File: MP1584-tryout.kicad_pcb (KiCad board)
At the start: 2 copper layers, 15 parts, among them J1 Conn_01x03_Female, U1 MP1584

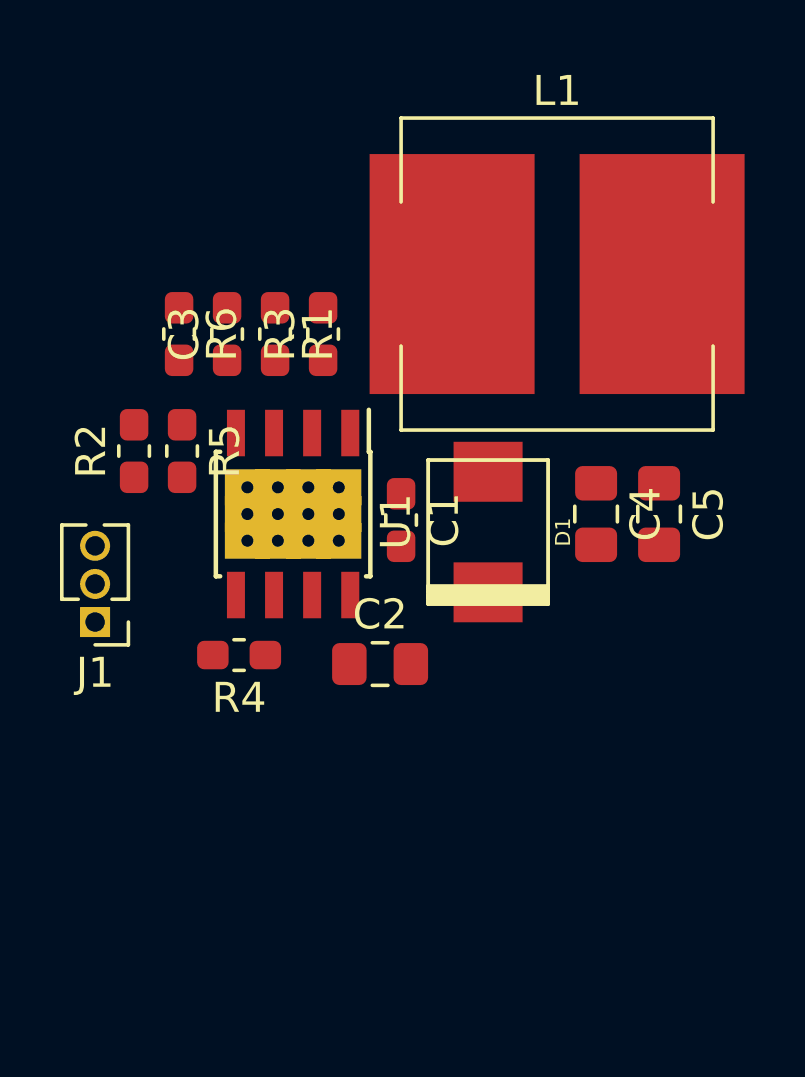
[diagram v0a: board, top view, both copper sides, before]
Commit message: final,
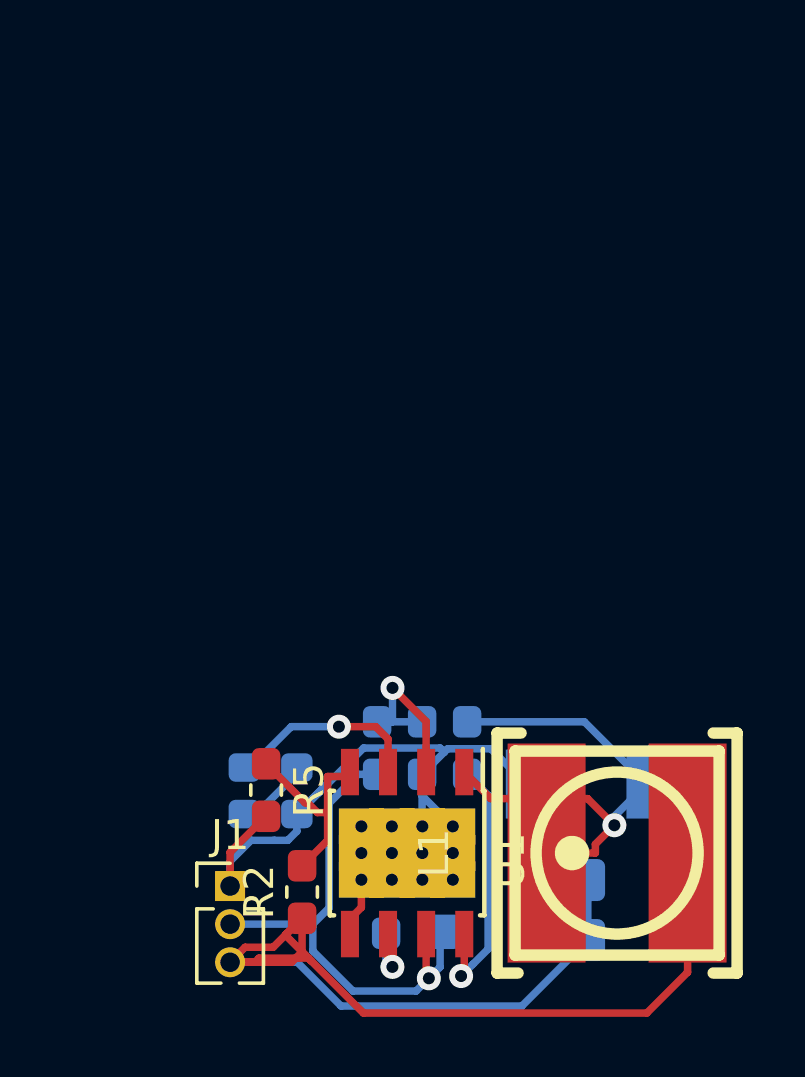
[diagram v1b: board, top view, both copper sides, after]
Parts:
- C1, C2, C3, C4, C5, D1, R1, R3, R4, R6: moved to B.Cu
- L1: footprint footprint-lib:L_SMD_ALL -> w_smd_inductors:inductor_smd_6.8x3.8mm
- U1: footprint footprint-lib:MP2303,SOIC-8_3.9x4.9mm_P1.27mm,thermal_via -> footprint-lib:MP1584,SOIC-8_3.9x4.9mm_P1.27mm,thermal_via
- moved L1 19.4 mm to (67.7, 63.4), turned to 90 degrees
- moved R6 16.3 mm to (56.1, 62.1), turned to 0 degrees
- moved R2 15.7 mm to (57.2, 64.7)
- moved C3 14.5 mm to (56.1, 60.5), turned to 0 degrees
- moved C4 14.3 mm to (65.7, 66.3), turned to 180 degrees
- moved R1 14.2 mm to (59.7, 59.9), turned to 90 degrees
- moved R3 14.2 mm to (61.2, 59.9), turned to 270 degrees
- moved C5 12.7 mm to (65.7, 64.3), turned to 180 degrees
- moved U1 11.9 mm to (60.7, 63.4)
- moved R5 11.6 mm to (56.0, 61.3)
- moved J1 9.88 mm to (54.8, 64.5), turned to 0 degrees
- moved R4 9.72 mm to (60.0, 65.2), turned to 90 degrees
- moved D1 9.14 mm to (67.0, 61.1), turned to 180 degrees
- moved C2 8.15 mm to (61.8, 65.0), turned to 90 degrees
- moved C1 7.91 mm to (62.7, 59.9)
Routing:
- net +5V: track 0.00 -> 45.0 mm
- net GND: track 0.00 -> 43.7 mm
- net Net-(C1-Pad1): track 0.00 -> 18.5 mm, vias 0 -> 1
- net Net-(C2-Pad1): track 0.00 -> 17.7 mm, vias 0 -> 1
- net Net-(C1-Pad2): track 0.00 -> 8.83 mm, vias 0 -> 1
- net Net-(R2-Pad2): track 0.00 -> 6.86 mm
- net Net-(C3-Pad1): track 0.00 -> 6.25 mm, vias 0 -> 1
- net Net-(R1-Pad2): track 0.00 -> 5.90 mm, vias 0 -> 1
- net Net-(R4-Pad1): track 0.00 -> 2.41 mm, vias 0 -> 1
- net Net-(C3-Pad2): track 0.00 -> 2.39 mm

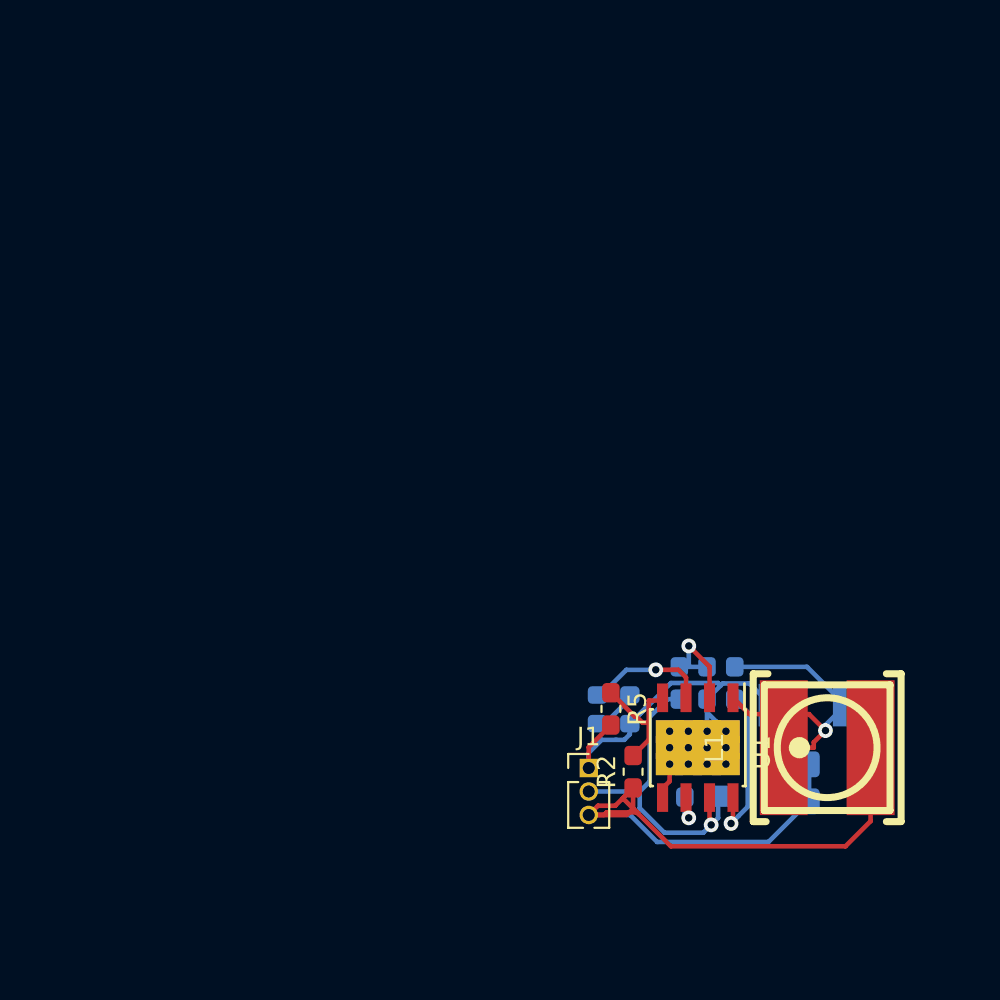
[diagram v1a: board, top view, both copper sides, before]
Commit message: update,
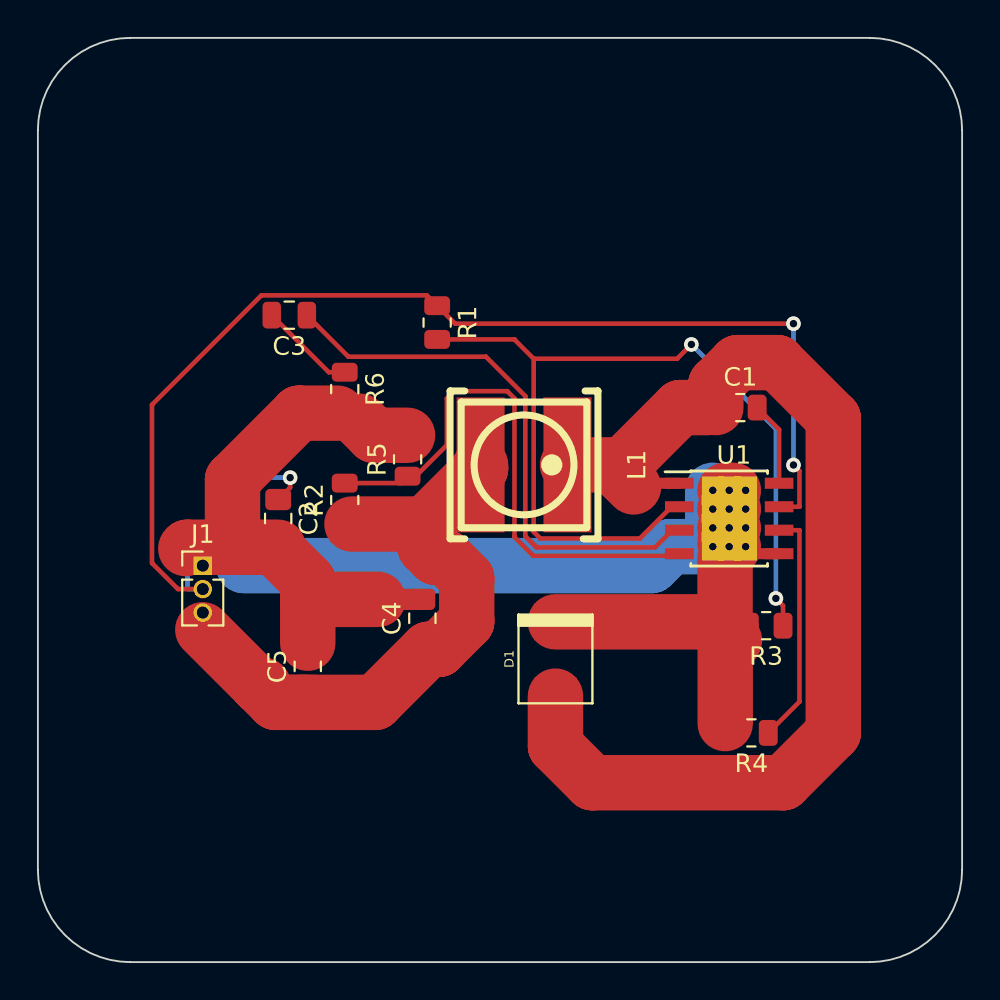
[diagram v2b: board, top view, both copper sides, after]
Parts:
- C1: value C104,0603 -> C104,0805; footprint Capacitor_SMD:C_0603_1608Metric_Pad1.05x0.95mm_HandSolder -> Resistor_SMD:R_0805_2012Metric; moved to F.Cu
- C2, C4, C5, D1: moved to F.Cu
- C3: value C151,0603 -> C151,0805; footprint Capacitor_SMD:C_0603_1608Metric_Pad1.05x0.95mm_HandSolder -> Capacitor_SMD:C_0805_2012Metric; moved to F.Cu
- R1, R4, R6: value R104,0603 -> R104,0805; footprint Resistor_SMD:R_0603_1608Metric_Pad1.05x0.95mm_HandSolder -> Resistor_SMD:R_0805_2012Metric; moved to F.Cu
- R2: value R224,0603 -> R224,0805; footprint Resistor_SMD:R_0603_1608Metric_Pad1.05x0.95mm_HandSolder -> Resistor_SMD:R_0805_2012Metric
- R3: value R240,0603 -> R240,0805; footprint Resistor_SMD:R_0603_1608Metric_Pad1.05x0.95mm_HandSolder -> Resistor_SMD:R_0805_2012Metric; moved to F.Cu
- R5: value R433,0603 -> R433,0805; footprint Resistor_SMD:R_0603_1608Metric_Pad1.05x0.95mm_HandSolder -> Resistor_SMD:R_0805_2012Metric
- moved C2 27.6 mm to (38.0, 51.0), turned to 270 degrees
- moved C3 27.0 mm to (38.6, 40.0), turned to 180 degrees
- moved C5 26.6 mm to (39.6, 59.0), turned to 90 degrees
- moved J1 23.6 mm to (33.9, 53.5)
- moved R1 23.5 mm to (46.6, 40.4), turned to 270 degrees
- moved R6 23.2 mm to (41.6, 44.0), turned to 270 degrees
- moved L1 22.4 mm to (51.3, 48.1), turned to 270 degrees
- moved C4 22.2 mm to (45.8, 56.4), turned to 90 degrees
- moved R2 21.4 mm to (41.6, 50.0)
- moved R5 17.4 mm to (45.0, 47.8), turned to 90 degrees
- moved C1 14.9 mm to (63.0, 45.0), turned to 0 degrees
- moved D1 14.2 mm to (53.0, 58.6), turned to 90 degrees
- moved U1 12.5 mm to (62.4, 51.0), turned to 0 degrees
- moved R3 4.46 mm to (64.4, 56.8), turned to 180 degrees
- moved R4 4.44 mm to (63.6, 62.6), turned to 180 degrees
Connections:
- net Net-(C1-Pad1) renamed /SW_OUT
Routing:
- net Net-(C2-Pad1): track 17.7 -> 72.3 mm, vias 1 -> 3
- net GND: track 43.7 -> 96.7 mm
- net Net-(R1-Pad2): track 5.90 -> 49.9 mm, vias 1 -> 2
- net /SW_OUT: track 18.5 -> 59.7 mm, vias 1 -> 0
- net Net-(C3-Pad1): track 6.25 -> 30.2 mm, vias 1 -> 0
- net Net-(R2-Pad2): track 6.86 -> 29.8 mm
- net Net-(R4-Pad1): track 2.41 -> 12.8 mm, vias 1 -> 0
- net +5V: track 45.0 -> 38.0 mm
- net Net-(C1-Pad2): track 8.83 -> 4.59 mm, vias 1 -> 0
- net Net-(C3-Pad2): track 2.39 -> 5.23 mm
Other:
- board outline added: 50 x 50 mm
- net class CURRENT_1A added: clearance 0.2, trace_width 3, via_dia 2, via_drill 1
